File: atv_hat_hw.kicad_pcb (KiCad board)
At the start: 2 copper layers, 84.1 x 83.9 mm, 51 parts, among them J1 GPIO_CONNECTOR, J10 conn_01x02_labeled, J11 conn_01x02_labeled, J12 conn_01x02_labeled, J2 conn_01x02_labeled, J3 conn_01x02_labeled, J4 conn_01x02_labeled, J5 conn_01x02_labeled, J6 conn_01x02_labeled, J7 enc28j60_hanrun, J8 conn_01x02_labeled, J9 conn_01x02_labeled, Q1 Q_NMOS_GDS, Q2 Q_NMOS_GDS, Q3 Q_NMOS_GDS, Q4 Q_NMOS_GDS, Q5 Q_NMOS_GDS, Q6 Q_NMOS_GDS, Q7 Q_NMOS_GDS, Q8 Q_NMOS_GDS, Q9 Q_NMOS_GDS

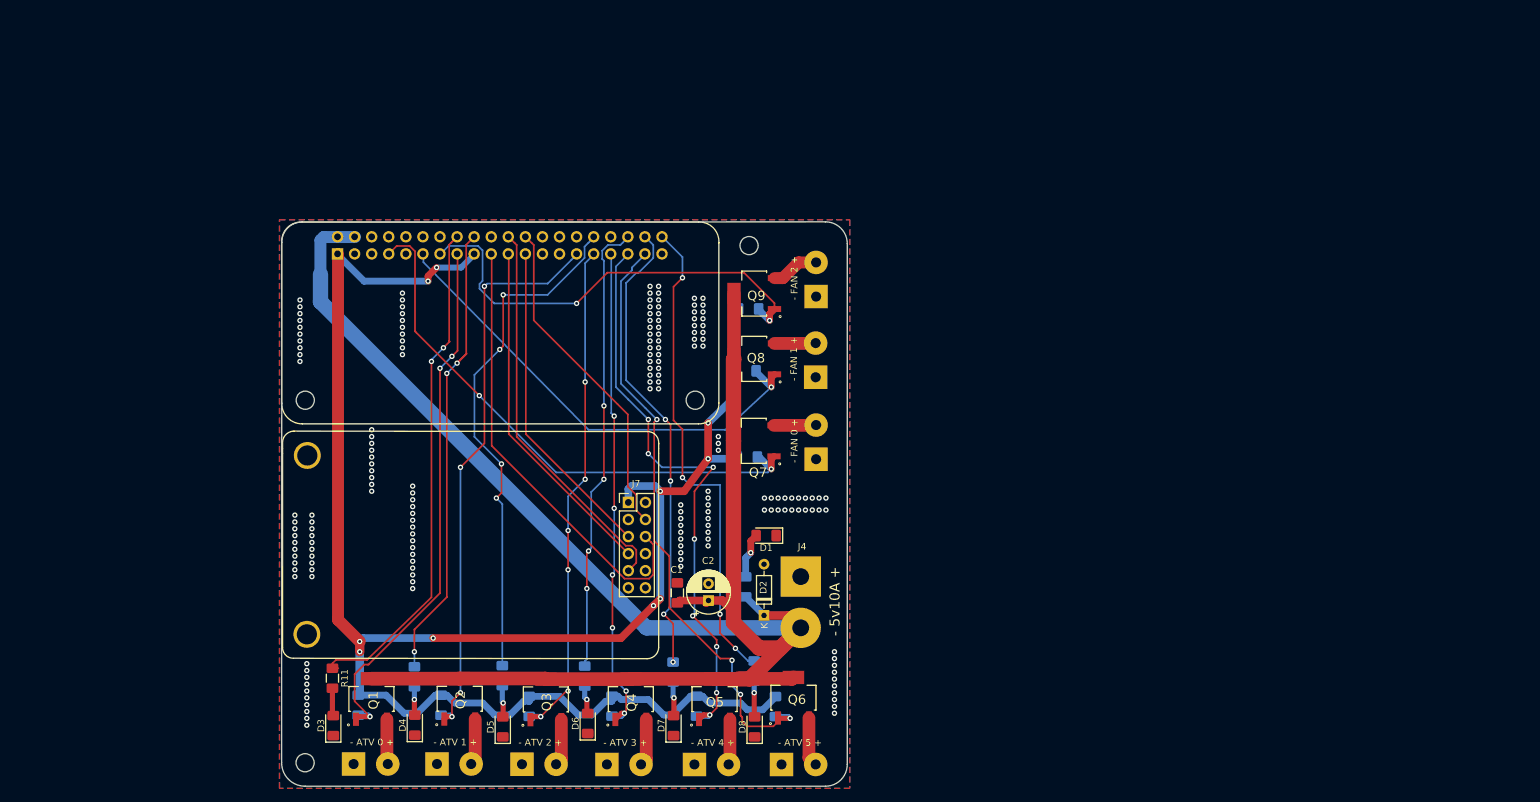
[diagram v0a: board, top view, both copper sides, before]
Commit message: plus board ready for routing
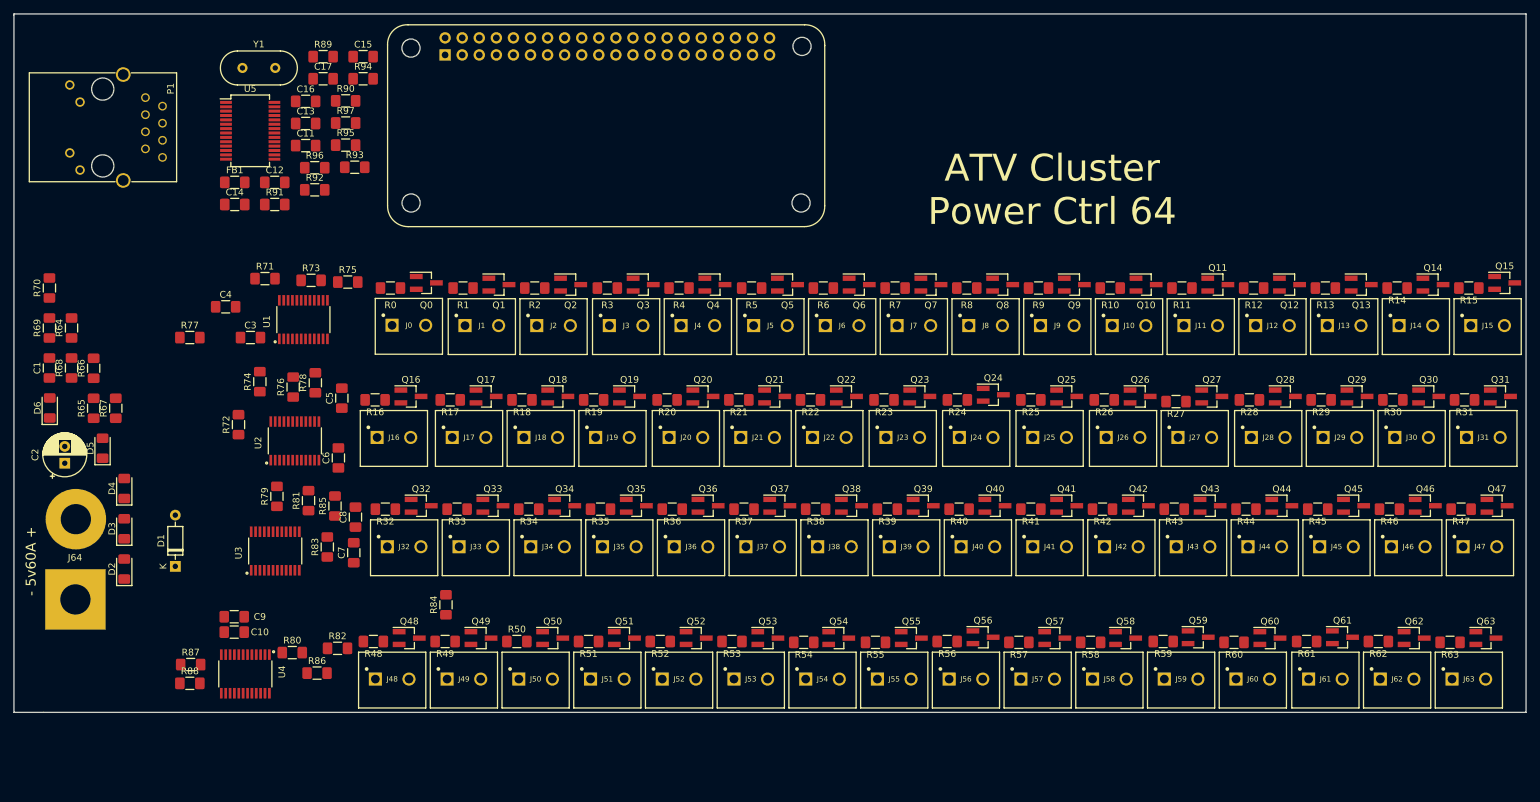
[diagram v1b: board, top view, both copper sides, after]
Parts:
- removed D7, D8: Green, LED_SMD:LED_1206_3216Metric_Pad1.42x1.75mm_HandSolder
- removed the H4 at (90.6, 129.6)
- added C10: 10u, Capacitor_SMD:C_1206_3216Metric_Pad1.42x1.75mm_HandSolder, F.Cu at (80.0, 107.9)
- added C11: 100n, Capacitor_SMD:C_1206_3216Metric_Pad1.42x1.75mm_HandSolder, F.Cu at (90.6, 37.8)
- added C12: 30p, Capacitor_SMD:C_1206_3216Metric_Pad1.42x1.75mm_HandSolder, F.Cu at (86.0, 43.3)
- added C13: 30p, Capacitor_SMD:C_1206_3216Metric_Pad1.42x1.75mm_HandSolder, F.Cu at (90.6, 34.5)
- added C14: 10u, Capacitor_SMD:C_1206_3216Metric_Pad1.42x1.75mm_HandSolder, F.Cu at (80.1, 46.6)
- added C15: 100n, Capacitor_SMD:C_1206_3216Metric_Pad1.42x1.75mm_HandSolder, F.Cu at (99.2, 24.6)
- added C16: 100n, Capacitor_SMD:C_1206_3216Metric_Pad1.42x1.75mm_HandSolder, F.Cu at (90.6, 31.2)
- added C17: 10u, Capacitor_SMD:C_1206_3216Metric_Pad1.42x1.75mm_HandSolder, F.Cu at (93.2, 27.9)
- added C3: 100n, Capacitor_SMD:C_1206_3216Metric_Pad1.42x1.75mm_HandSolder, F.Cu at (82.4, 66.4)
- added C4: 10u, Capacitor_SMD:C_1206_3216Metric_Pad1.42x1.75mm_HandSolder, F.Cu at (78.7, 61.8)
- added C5: 100n, Capacitor_SMD:C_1206_3216Metric_Pad1.42x1.75mm_HandSolder, F.Cu at (96.0, 75.4)
- added C6: 10u, Capacitor_SMD:C_1206_3216Metric_Pad1.42x1.75mm_HandSolder, F.Cu at (95.5, 84.3)
- added C7: 100n, Capacitor_SMD:C_1206_3216Metric_Pad1.42x1.75mm_HandSolder, F.Cu at (97.8, 98.4)
- added C8: 10u, Capacitor_SMD:C_1206_3216Metric_Pad1.42x1.75mm_HandSolder, F.Cu at (98.0, 93.1)
- added C9: 100n, Capacitor_SMD:C_1206_3216Metric_Pad1.42x1.75mm_HandSolder, F.Cu at (80.0, 110.2)
- added FB1: 80mA, Inductor_SMD:L_1206_3216Metric_Pad1.42x1.75mm_HandSolder, F.Cu at (80.1, 43.3)
- added H1: MountingHole, lib:MountingHole_2.7mm_M2.5_uHAT_RPi, F.Cu at (106.3, 23.3)
- added J0: phoenix_1935161, lib:PHOENIX_1935161, F.Cu at (106.0, 64.6)
- added J13: phoenix_1935161, lib:PHOENIX_1935161, F.Cu at (245.1, 64.6)
- added J14: phoenix_1935161, lib:PHOENIX_1935161, F.Cu at (255.8, 64.6)
- added J15: phoenix_1935161, lib:PHOENIX_1935161, F.Cu at (266.4, 64.6)
- added J16: phoenix_1935161, lib:PHOENIX_1935161, F.Cu at (103.8, 81.2)
- added J17: phoenix_1935161, lib:PHOENIX_1935161, F.Cu at (114.9, 81.2)
- added J18: phoenix_1935161, lib:PHOENIX_1935161, F.Cu at (125.6, 81.2)
- added J19: phoenix_1935161, lib:PHOENIX_1935161, F.Cu at (136.3, 81.2)
- added J20: phoenix_1935161, lib:PHOENIX_1935161, F.Cu at (147.2, 81.2)
- added J21: phoenix_1935161, lib:PHOENIX_1935161, F.Cu at (157.9, 81.2)
- added J22: phoenix_1935161, lib:PHOENIX_1935161, F.Cu at (168.5, 81.2)
- added J23: phoenix_1935161, lib:PHOENIX_1935161, F.Cu at (179.5, 81.2)
- added J24: phoenix_1935161, lib:PHOENIX_1935161, F.Cu at (190.4, 81.2)
- added J25: phoenix_1935161, lib:PHOENIX_1935161, F.Cu at (201.3, 81.2)
- added J26: phoenix_1935161, lib:PHOENIX_1935161, F.Cu at (212.2, 81.2)
- added J27: phoenix_1935161, lib:PHOENIX_1935161, F.Cu at (222.9, 81.2)
- added J28: phoenix_1935161, lib:PHOENIX_1935161, F.Cu at (233.8, 81.2)
- added J29: phoenix_1935161, lib:PHOENIX_1935161, F.Cu at (244.5, 81.2)
- added J30: phoenix_1935161, lib:PHOENIX_1935161, F.Cu at (255.1, 81.2)
- added J31: phoenix_1935161, lib:PHOENIX_1935161, F.Cu at (265.8, 81.2)
- added J32: phoenix_1935161, lib:PHOENIX_1935161, F.Cu at (105.3, 97.5)
- added J33: phoenix_1935161, lib:PHOENIX_1935161, F.Cu at (116.0, 97.5)
- added J34: phoenix_1935161, lib:PHOENIX_1935161, F.Cu at (126.6, 97.5)
- added J35: phoenix_1935161, lib:PHOENIX_1935161, F.Cu at (137.3, 97.5)
- added J36: phoenix_1935161, lib:PHOENIX_1935161, F.Cu at (148.0, 97.5)
- added J37: phoenix_1935161, lib:PHOENIX_1935161, F.Cu at (158.6, 97.5)
- added J38: phoenix_1935161, lib:PHOENIX_1935161, F.Cu at (169.3, 97.5)
- added J39: phoenix_1935161, lib:PHOENIX_1935161, F.Cu at (180.0, 97.5)
- added J40: phoenix_1935161, lib:PHOENIX_1935161, F.Cu at (190.6, 97.5)
- added J41: phoenix_1935161, lib:PHOENIX_1935161, F.Cu at (201.3, 97.5)
- added J42: phoenix_1935161, lib:PHOENIX_1935161, F.Cu at (212.0, 97.5)
- added J43: phoenix_1935161, lib:PHOENIX_1935161, F.Cu at (222.6, 97.5)
- added J44: phoenix_1935161, lib:PHOENIX_1935161, F.Cu at (233.3, 97.5)
- added J45: phoenix_1935161, lib:PHOENIX_1935161, F.Cu at (244.0, 97.5)
- added J46: phoenix_1935161, lib:PHOENIX_1935161, F.Cu at (254.6, 97.5)
- added J47: phoenix_1935161, lib:PHOENIX_1935161, F.Cu at (265.3, 97.5)
- added J48: phoenix_1935161, lib:PHOENIX_1935161, F.Cu at (103.5, 117.2)
- added J49: phoenix_1935161, lib:PHOENIX_1935161, F.Cu at (114.2, 117.2)
- added J50: phoenix_1935161, lib:PHOENIX_1935161, F.Cu at (124.8, 117.2)
- added J51: phoenix_1935161, lib:PHOENIX_1935161, F.Cu at (135.5, 117.2)
- added J52: phoenix_1935161, lib:PHOENIX_1935161, F.Cu at (146.2, 117.2)
- added J53: phoenix_1935161, lib:PHOENIX_1935161, F.Cu at (156.8, 117.2)
- added J54: phoenix_1935161, lib:PHOENIX_1935161, F.Cu at (167.5, 117.2)
- added J55: phoenix_1935161, lib:PHOENIX_1935161, F.Cu at (178.2, 117.2)
- added J56: phoenix_1935161, lib:PHOENIX_1935161, F.Cu at (188.8, 117.2)
- added J57: phoenix_1935161, lib:PHOENIX_1935161, F.Cu at (199.5, 117.2)
- added J58: phoenix_1935161, lib:PHOENIX_1935161, F.Cu at (210.2, 117.2)
- added J59: phoenix_1935161, lib:PHOENIX_1935161, F.Cu at (220.9, 117.2)
- added J60: phoenix_1935161, lib:PHOENIX_1935161, F.Cu at (231.5, 117.2)
- added J61: phoenix_1935161, lib:PHOENIX_1935161, F.Cu at (242.3, 117.2)
- added J62: phoenix_1935161, lib:PHOENIX_1935161, F.Cu at (253.0, 117.2)
- added J63: phoenix_1935161, lib:PHOENIX_1935161, F.Cu at (263.7, 117.2)
- added J64: phoenix_1935161, lib:SolderWirePad_1x02_P9.0mm_Drill4.5mm, F.Cu at (56.5, 105.3)
- added J65: GPIO_CONNECTOR, lib:PinSocket_2x20_P2.54mm_Vertical_Centered_Anchor, B.Cu at (135.5, 23.1)
- added P1: RB1-125BAG1A, WIZNET_RB1-125BAG1A, F.Cu at (60.5, 35.1)
- added Q0: Q_NMOS_GSD, Package_TO_SOT_SMD:SOT-23_Handsoldering, F.Cu at (108.6, 58.2)
- added Q10: Q_NMOS_GSD, Package_TO_SOT_SMD:SOT-23_Handsoldering, F.Cu at (215.6, 58.5)
- added Q11: Q_NMOS_GSD, Package_TO_SOT_SMD:SOT-23_Handsoldering, F.Cu at (226.3, 58.5)
- added Q12: Q_NMOS_GSD, Package_TO_SOT_SMD:SOT-23_Handsoldering, F.Cu at (237.0, 58.5)
- added Q13: Q_NMOS_GSD, Package_TO_SOT_SMD:SOT-23_Handsoldering, F.Cu at (247.7, 58.5)
- added Q14: Q_NMOS_GSD, Package_TO_SOT_SMD:SOT-23_Handsoldering, F.Cu at (258.3, 58.5)
- added Q15: Q_NMOS_GSD, Package_TO_SOT_SMD:SOT-23_Handsoldering, F.Cu at (269.0, 58.2)
- added Q16: Q_NMOS_GSD, Package_TO_SOT_SMD:SOT-23_Handsoldering, F.Cu at (106.3, 75.1)
- added Q17: Q_NMOS_GSD, Package_TO_SOT_SMD:SOT-23_Handsoldering, F.Cu at (117.5, 75.1)
- added Q18: Q_NMOS_GSD, Package_TO_SOT_SMD:SOT-23_Handsoldering, F.Cu at (128.1, 75.1)
- added Q19: Q_NMOS_GSD, Package_TO_SOT_SMD:SOT-23_Handsoldering, F.Cu at (138.8, 75.1)
- added Q20: Q_NMOS_GSD, Package_TO_SOT_SMD:SOT-23_Handsoldering, F.Cu at (149.7, 75.1)
- added Q21: Q_NMOS_GSD, Package_TO_SOT_SMD:SOT-23_Handsoldering, F.Cu at (160.4, 75.1)
- added Q22: Q_NMOS_GSD, Package_TO_SOT_SMD:SOT-23_Handsoldering, F.Cu at (171.1, 75.1)
- added Q23: Q_NMOS_GSD, Package_TO_SOT_SMD:SOT-23_Handsoldering, F.Cu at (182.0, 75.1)
- added Q24: Q_NMOS_GSD, Package_TO_SOT_SMD:SOT-23_Handsoldering, F.Cu at (192.9, 74.9)
- added Q25: Q_NMOS_GSD, Package_TO_SOT_SMD:SOT-23_Handsoldering, F.Cu at (203.8, 75.1)
- added Q26: Q_NMOS_GSD, Package_TO_SOT_SMD:SOT-23_Handsoldering, F.Cu at (214.8, 75.1)
- added Q27: Q_NMOS_GSD, Package_TO_SOT_SMD:SOT-23_Handsoldering, F.Cu at (225.4, 75.1)
- added Q28: Q_NMOS_GSD, Package_TO_SOT_SMD:SOT-23_Handsoldering, F.Cu at (236.3, 75.1)
- added Q29: Q_NMOS_GSD, Package_TO_SOT_SMD:SOT-23_Handsoldering, F.Cu at (247.0, 75.1)
- added Q30: Q_NMOS_GSD, Package_TO_SOT_SMD:SOT-23_Handsoldering, F.Cu at (257.7, 75.1)
- added Q31: Q_NMOS_GSD, Package_TO_SOT_SMD:SOT-23_Handsoldering, F.Cu at (268.4, 75.1)
- added Q32: Q_NMOS_GSD, Package_TO_SOT_SMD:SOT-23_Handsoldering, F.Cu at (107.8, 91.4)
- added Q33: Q_NMOS_GSD, Package_TO_SOT_SMD:SOT-23_Handsoldering, F.Cu at (118.5, 91.4)
- added Q34: Q_NMOS_GSD, Package_TO_SOT_SMD:SOT-23_Handsoldering, F.Cu at (129.2, 91.4)
- added Q35: Q_NMOS_GSD, Package_TO_SOT_SMD:SOT-23_Handsoldering, F.Cu at (139.8, 91.4)
- added Q36: Q_NMOS_GSD, Package_TO_SOT_SMD:SOT-23_Handsoldering, F.Cu at (150.5, 91.4)
- added Q37: Q_NMOS_GSD, Package_TO_SOT_SMD:SOT-23_Handsoldering, F.Cu at (161.2, 91.4)
- added Q38: Q_NMOS_GSD, Package_TO_SOT_SMD:SOT-23_Handsoldering, F.Cu at (171.8, 91.4)
- added Q39: Q_NMOS_GSD, Package_TO_SOT_SMD:SOT-23_Handsoldering, F.Cu at (182.5, 91.4)
- added Q40: Q_NMOS_GSD, Package_TO_SOT_SMD:SOT-23_Handsoldering, F.Cu at (193.2, 91.4)
- added Q41: Q_NMOS_GSD, Package_TO_SOT_SMD:SOT-23_Handsoldering, F.Cu at (203.8, 91.4)
- added Q42: Q_NMOS_GSD, Package_TO_SOT_SMD:SOT-23_Handsoldering, F.Cu at (214.5, 91.4)
- added Q43: Q_NMOS_GSD, Package_TO_SOT_SMD:SOT-23_Handsoldering, F.Cu at (225.2, 91.4)
- added Q44: Q_NMOS_GSD, Package_TO_SOT_SMD:SOT-23_Handsoldering, F.Cu at (235.8, 91.4)
- added Q45: Q_NMOS_GSD, Package_TO_SOT_SMD:SOT-23_Handsoldering, F.Cu at (246.5, 91.4)
- added Q46: Q_NMOS_GSD, Package_TO_SOT_SMD:SOT-23_Handsoldering, F.Cu at (257.2, 91.4)
- added Q47: Q_NMOS_GSD, Package_TO_SOT_SMD:SOT-23_Handsoldering, F.Cu at (267.8, 91.4)
- added Q48: Q_NMOS_GSD, Package_TO_SOT_SMD:SOT-23_Handsoldering, F.Cu at (106.0, 111.1)
- added Q49: Q_NMOS_GSD, Package_TO_SOT_SMD:SOT-23_Handsoldering, F.Cu at (116.7, 111.1)
- added Q50: Q_NMOS_GSD, Package_TO_SOT_SMD:SOT-23_Handsoldering, F.Cu at (127.4, 111.1)
- added Q51: Q_NMOS_GSD, Package_TO_SOT_SMD:SOT-23_Handsoldering, F.Cu at (138.1, 111.1)
- added Q52: Q_NMOS_GSD, Package_TO_SOT_SMD:SOT-23_Handsoldering, F.Cu at (148.7, 111.1)
- added Q53: Q_NMOS_GSD, Package_TO_SOT_SMD:SOT-23_Handsoldering, F.Cu at (159.4, 111.1)
- added Q54: Q_NMOS_GSD, Package_TO_SOT_SMD:SOT-23_Handsoldering, F.Cu at (169.9, 111.1)
- added Q55: Q_NMOS_GSD, Package_TO_SOT_SMD:SOT-23_Handsoldering, F.Cu at (180.7, 111.1)
- added Q56: Q_NMOS_GSD, Package_TO_SOT_SMD:SOT-23_Handsoldering, F.Cu at (191.4, 111.0)
- added Q57: Q_NMOS_GSD, Package_TO_SOT_SMD:SOT-23_Handsoldering, F.Cu at (202.1, 111.1)
- added Q58: Q_NMOS_GSD, Package_TO_SOT_SMD:SOT-23_Handsoldering, F.Cu at (212.6, 111.1)
- added Q59: Q_NMOS_GSD, Package_TO_SOT_SMD:SOT-23_Handsoldering, F.Cu at (223.4, 111.0)
- added Q60: Q_NMOS_GSD, Package_TO_SOT_SMD:SOT-23_Handsoldering, F.Cu at (234.1, 111.1)
- added Q61: Q_NMOS_GSD, Package_TO_SOT_SMD:SOT-23_Handsoldering, F.Cu at (244.9, 111.0)
- added Q62: Q_NMOS_GSD, Package_TO_SOT_SMD:SOT-23_Handsoldering, F.Cu at (255.5, 111.1)
- added Q63: Q_NMOS_GSD, Package_TO_SOT_SMD:SOT-23_Handsoldering, F.Cu at (266.2, 111.1)
- added R0: 10k, Resistor_SMD:R_1206_3216Metric_Pad1.42x1.75mm_HandSolder, F.Cu at (103.3, 59.0)
- added R17: 10k, Resistor_SMD:R_1206_3216Metric_Pad1.42x1.75mm_HandSolder, F.Cu at (112.1, 75.6)
- added R18: 10k, Resistor_SMD:R_1206_3216Metric_Pad1.42x1.75mm_HandSolder, F.Cu at (122.8, 75.6)
- added R19: 10k, Resistor_SMD:R_1206_3216Metric_Pad1.42x1.75mm_HandSolder, F.Cu at (133.5, 75.6)
- added R20: 10k, Resistor_SMD:R_1206_3216Metric_Pad1.42x1.75mm_HandSolder, F.Cu at (144.4, 75.6)
- added R21: 10k, Resistor_SMD:R_1206_3216Metric_Pad1.42x1.75mm_HandSolder, F.Cu at (155.1, 75.6)
- added R22: 10k, Resistor_SMD:R_1206_3216Metric_Pad1.42x1.75mm_HandSolder, F.Cu at (165.7, 75.6)
- added R23: 10k, Resistor_SMD:R_1206_3216Metric_Pad1.42x1.75mm_HandSolder, F.Cu at (176.7, 75.6)
- added R24: 10k, Resistor_SMD:R_1206_3216Metric_Pad1.42x1.75mm_HandSolder, F.Cu at (187.6, 75.6)
- added R25: 10k, Resistor_SMD:R_1206_3216Metric_Pad1.42x1.75mm_HandSolder, F.Cu at (198.5, 75.6)
- added R26: 10k, Resistor_SMD:R_1206_3216Metric_Pad1.42x1.75mm_HandSolder, F.Cu at (209.4, 75.6)
- added R27: 10k, Resistor_SMD:R_1206_3216Metric_Pad1.42x1.75mm_HandSolder, F.Cu at (220.1, 75.9)
- added R28: 10k, Resistor_SMD:R_1206_3216Metric_Pad1.42x1.75mm_HandSolder, F.Cu at (231.0, 75.6)
- added R29: 10k, Resistor_SMD:R_1206_3216Metric_Pad1.42x1.75mm_HandSolder, F.Cu at (241.7, 75.6)
- added R30: 10k, Resistor_SMD:R_1206_3216Metric_Pad1.42x1.75mm_HandSolder, F.Cu at (252.3, 75.6)
- added R31: 10k, Resistor_SMD:R_1206_3216Metric_Pad1.42x1.75mm_HandSolder, F.Cu at (263.0, 75.6)
- added R32: 10k, Resistor_SMD:R_1206_3216Metric_Pad1.42x1.75mm_HandSolder, F.Cu at (102.5, 91.9)
- added R33: 10k, Resistor_SMD:R_1206_3216Metric_Pad1.42x1.75mm_HandSolder, F.Cu at (113.2, 91.9)
- added R34: 10k, Resistor_SMD:R_1206_3216Metric_Pad1.42x1.75mm_HandSolder, F.Cu at (123.8, 91.9)
- added R35: 10k, Resistor_SMD:R_1206_3216Metric_Pad1.42x1.75mm_HandSolder, F.Cu at (134.5, 91.9)
- added R36: 10k, Resistor_SMD:R_1206_3216Metric_Pad1.42x1.75mm_HandSolder, F.Cu at (145.2, 91.9)
- added R37: 10k, Resistor_SMD:R_1206_3216Metric_Pad1.42x1.75mm_HandSolder, F.Cu at (155.8, 91.9)
- added R38: 10k, Resistor_SMD:R_1206_3216Metric_Pad1.42x1.75mm_HandSolder, F.Cu at (166.5, 91.9)
- added R39: 10k, Resistor_SMD:R_1206_3216Metric_Pad1.42x1.75mm_HandSolder, F.Cu at (177.2, 91.9)
- added R40: 10k, Resistor_SMD:R_1206_3216Metric_Pad1.42x1.75mm_HandSolder, F.Cu at (187.8, 91.9)
- added R41: 10k, Resistor_SMD:R_1206_3216Metric_Pad1.42x1.75mm_HandSolder, F.Cu at (198.5, 91.9)
- added R42: 10k, Resistor_SMD:R_1206_3216Metric_Pad1.42x1.75mm_HandSolder, F.Cu at (209.2, 91.9)
- added R43: 10k, Resistor_SMD:R_1206_3216Metric_Pad1.42x1.75mm_HandSolder, F.Cu at (219.8, 91.9)
- added R44: 10k, Resistor_SMD:R_1206_3216Metric_Pad1.42x1.75mm_HandSolder, F.Cu at (230.5, 91.9)
- added R45: 10k, Resistor_SMD:R_1206_3216Metric_Pad1.42x1.75mm_HandSolder, F.Cu at (241.2, 91.9)
- added R46: 10k, Resistor_SMD:R_1206_3216Metric_Pad1.42x1.75mm_HandSolder, F.Cu at (251.8, 91.9)
- added R47: 10k, Resistor_SMD:R_1206_3216Metric_Pad1.42x1.75mm_HandSolder, F.Cu at (262.5, 91.9)
- added R48: 10k, Resistor_SMD:R_1206_3216Metric_Pad1.42x1.75mm_HandSolder, F.Cu at (100.7, 111.6)
- added R49: 10k, Resistor_SMD:R_1206_3216Metric_Pad1.42x1.75mm_HandSolder, F.Cu at (111.4, 111.6)
- added R50: 10k, Resistor_SMD:R_1206_3216Metric_Pad1.42x1.75mm_HandSolder, F.Cu at (122.0, 111.6)
- added R51: 10k, Resistor_SMD:R_1206_3216Metric_Pad1.42x1.75mm_HandSolder, F.Cu at (132.7, 111.6)
- added R52: 10k, Resistor_SMD:R_1206_3216Metric_Pad1.42x1.75mm_HandSolder, F.Cu at (143.4, 111.6)
- added R53: 10k, Resistor_SMD:R_1206_3216Metric_Pad1.42x1.75mm_HandSolder, F.Cu at (154.1, 111.6)
- added R54: 10k, Resistor_SMD:R_1206_3216Metric_Pad1.42x1.75mm_HandSolder, F.Cu at (164.7, 111.7)
- added R55: 10k, Resistor_SMD:R_1206_3216Metric_Pad1.42x1.75mm_HandSolder, F.Cu at (175.4, 111.7)
- added R56: 10k, Resistor_SMD:R_1206_3216Metric_Pad1.42x1.75mm_HandSolder, F.Cu at (186.1, 111.6)
- added R57: 10k, Resistor_SMD:R_1206_3216Metric_Pad1.42x1.75mm_HandSolder, F.Cu at (196.7, 111.7)
- added R58: 10k, Resistor_SMD:R_1206_3216Metric_Pad1.42x1.75mm_HandSolder, F.Cu at (207.4, 111.7)
- added R59: 10k, Resistor_SMD:R_1206_3216Metric_Pad1.42x1.75mm_HandSolder, F.Cu at (218.2, 111.6)
- added R60: 10k, Resistor_SMD:R_1206_3216Metric_Pad1.42x1.75mm_HandSolder, F.Cu at (228.7, 111.7)
- added R61: 10k, Resistor_SMD:R_1206_3216Metric_Pad1.42x1.75mm_HandSolder, F.Cu at (239.5, 111.6)
- added R62: 10k, Resistor_SMD:R_1206_3216Metric_Pad1.42x1.75mm_HandSolder, F.Cu at (250.2, 111.6)
- added R63: 10k, Resistor_SMD:R_1206_3216Metric_Pad1.42x1.75mm_HandSolder, F.Cu at (260.9, 111.7)
- added R64: 220, Resistor_SMD:R_1206_3216Metric_Pad1.42x1.75mm_HandSolder, F.Cu at (55.8, 65.0)
- added R65: 10k, Resistor_SMD:R_1206_3216Metric_Pad1.42x1.75mm_HandSolder, F.Cu at (59.1, 76.9)
- added R66: 10k, Resistor_SMD:R_1206_3216Metric_Pad1.42x1.75mm_HandSolder, F.Cu at (59.1, 70.9)
- added R67: 220, Resistor_SMD:R_1206_3216Metric_Pad1.42x1.75mm_HandSolder, F.Cu at (62.4, 76.9)
- added R68: 220, Resistor_SMD:R_1206_3216Metric_Pad1.42x1.75mm_HandSolder, F.Cu at (55.8, 70.9)
- added R69: 220, Resistor_SMD:R_1206_3216Metric_Pad1.42x1.75mm_HandSolder, F.Cu at (52.5, 65.0)
- added R70: 220, Resistor_SMD:R_1206_3216Metric_Pad1.42x1.75mm_HandSolder, F.Cu at (52.5, 59.0)
- added R71: 10k, Resistor_SMD:R_1206_3216Metric_Pad1.42x1.75mm_HandSolder, F.Cu at (84.6, 57.6)
- added R72: 10k, Resistor_SMD:R_1206_3216Metric_Pad1.42x1.75mm_HandSolder, F.Cu at (80.6, 79.3)
- added R73: 10k, Resistor_SMD:R_1206_3216Metric_Pad1.42x1.75mm_HandSolder, F.Cu at (91.4, 57.9)
- added R74: 10k, Resistor_SMD:R_1206_3216Metric_Pad1.42x1.75mm_HandSolder, F.Cu at (83.8, 72.9)
- added R75: 10k, Resistor_SMD:R_1206_3216Metric_Pad1.42x1.75mm_HandSolder, F.Cu at (96.9, 58.1)
- added R76: 10k, Resistor_SMD:R_1206_3216Metric_Pad1.42x1.75mm_HandSolder, F.Cu at (88.8, 73.7)
- added R77: 10k, Resistor_SMD:R_1206_3216Metric_Pad1.42x1.75mm_HandSolder, F.Cu at (73.4, 66.4)
- added R78: 10k, Resistor_SMD:R_1206_3216Metric_Pad1.42x1.75mm_HandSolder, F.Cu at (92.1, 73.1)
- added R79: 10k, Resistor_SMD:R_1206_3216Metric_Pad1.42x1.75mm_HandSolder, F.Cu at (86.4, 90.0)
- added R80: 10k, Resistor_SMD:R_1206_3216Metric_Pad1.42x1.75mm_HandSolder, F.Cu at (88.6, 113.2)
- added R81: 10k, Resistor_SMD:R_1206_3216Metric_Pad1.42x1.75mm_HandSolder, F.Cu at (91.1, 90.6)
- added R82: 10k, Resistor_SMD:R_1206_3216Metric_Pad1.42x1.75mm_HandSolder, F.Cu at (95.4, 112.6)
- added R83: 10k, Resistor_SMD:R_1206_3216Metric_Pad1.42x1.75mm_HandSolder, F.Cu at (93.9, 97.5)
- added R84: 10k, Resistor_SMD:R_1206_3216Metric_Pad1.42x1.75mm_HandSolder, F.Cu at (111.5, 106.1)
- added R85: 10k, Resistor_SMD:R_1206_3216Metric_Pad1.42x1.75mm_HandSolder, F.Cu at (95.0, 91.4)
- added R86: 10k, Resistor_SMD:R_1206_3216Metric_Pad1.42x1.75mm_HandSolder, F.Cu at (92.3, 116.3)
- added R87: 10k, Resistor_SMD:R_1206_3216Metric_Pad1.42x1.75mm_HandSolder, F.Cu at (73.5, 115.0)
- added R88: 10k, Resistor_SMD:R_1206_3216Metric_Pad1.42x1.75mm_HandSolder, F.Cu at (73.4, 117.8)
- added R89: 10k, Resistor_SMD:R_1206_3216Metric_Pad1.42x1.75mm_HandSolder, F.Cu at (93.2, 24.6)
- added R90: 10k, Resistor_SMD:R_1206_3216Metric_Pad1.42x1.75mm_HandSolder, F.Cu at (96.6, 31.2)
- added R91: 10k, Resistor_SMD:R_1206_3216Metric_Pad1.42x1.75mm_HandSolder, F.Cu at (86.0, 46.6)
- added R92: 10k, Resistor_SMD:R_1206_3216Metric_Pad1.42x1.75mm_HandSolder, F.Cu at (92.0, 44.4)
- added R93: 49.9, Resistor_SMD:R_1206_3216Metric_Pad1.42x1.75mm_HandSolder, F.Cu at (97.9, 41.0)
- added R94: 49.9, Resistor_SMD:R_1206_3216Metric_Pad1.42x1.75mm_HandSolder, F.Cu at (99.2, 27.9)
- added R95: 49.9, Resistor_SMD:R_1206_3216Metric_Pad1.42x1.75mm_HandSolder, F.Cu at (96.6, 37.8)
- added R96: 2.32k, Resistor_SMD:R_1206_3216Metric_Pad1.42x1.75mm_HandSolder, F.Cu at (92.0, 41.1)
- added R97: 49.9, Resistor_SMD:R_1206_3216Metric_Pad1.42x1.75mm_HandSolder, F.Cu at (96.6, 34.5)
- added U1: PCA9552PW,118, lib:SOP65P640X110-24N, F.Cu at (90.3, 63.7)
- added U2: PCA9552PW,118, lib:SOP65P640X110-24N, F.Cu at (89.0, 81.7)
- added U3: PCA9552PW,118, lib:SOP65P640X110-24N, F.Cu at (86.1, 98.1)
- added U4: PCA9552PW,118, lib:SOP65P640X110-24N, F.Cu at (81.7, 116.4)
- added U5: ENC28J60x-SS, Package_SO:SSOP-28_5.3x10.2mm_P0.65mm, F.Cu at (82.4, 35.6)
- added Y1: Crystal, Crystal:Crystal_HC49-4H_Vertical, F.Cu at (81.2, 26.3)
- D1: value Blue -> 5.6v; footprint LED_SMD:LED_1206_3216Metric_Pad1.42x1.75mm_HandSolder -> Diode_THT:D_DO-35_SOD27_P7.62mm_Horizontal
- D2: value 5.6v -> Blue; footprint Diode_THT:D_DO-35_SOD27_P7.62mm_Horizontal -> LED_SMD:LED_1206_3216Metric_Pad1.42x1.75mm_HandSolder
- J1: value GPIO_CONNECTOR -> phoenix_1935161; footprint lib:PinSocket_2x20_P2.54mm_Vertical_Centered_Anchor -> lib:PHOENIX_1935161; moved to F.Cu
- J10, J11, J12, J2, J3, J5, J6, J8, J9: value conn_01x02_labeled -> phoenix_1935161; footprint lib:SolderWirePad_1x02_P5.08mm_Drill1.5mm_labeled -> lib:PHOENIX_1935161
- J4: value conn_01x02_labeled -> phoenix_1935161; footprint Connector_Wire:SolderWirePad_1x02_P7.62mm_Drill2.5mm -> lib:PHOENIX_1935161
- J7: value enc28j60_hanrun -> phoenix_1935161; footprint lib:enc28j60_hanrun -> lib:PHOENIX_1935161
- Q1, Q2, Q3, Q4, Q5, Q6, Q7, Q8, Q9: value Q_NMOS_GDS -> Q_NMOS_GSD; footprint lib:SOT230P700X180-3N -> Package_TO_SOT_SMD:SOT-23_Handsoldering
- R1, R10, R2, R4, R5, R6, R7, R8, R9: moved to F.Cu
- R11: value 220 -> 10k
- R12, R13, R14, R15, R16, R3: value 220 -> 10k; moved to F.Cu
- moved R11 139.1 mm to (221.0, 59.0), turned to 180 degrees
- moved R12 137.6 mm to (231.6, 59.0), turned to 180 degrees
- moved R13 135.3 mm to (242.3, 59.0), turned to 180 degrees
- moved R14 133.9 mm to (253.0, 59.0), turned to 180 degrees
- moved R15 131.4 mm to (263.7, 59.0), turned to 180 degrees
- moved C1 99.2 mm to (52.5, 70.9), turned to 90 degrees
- moved C2 97.9 mm to (54.8, 85.1)
- moved D2 95.4 mm to (63.7, 100.8)
- moved D6 92.8 mm to (52.6, 76.8)
- moved D1 88.0 mm to (71.2, 100.4), turned to 90 degrees
- moved J8 78.3 mm to (191.8, 64.6)
- moved J9 77.1 mm to (202.4, 64.6)
- moved J5 75.0 mm to (159.8, 64.6)
- moved J6 74.1 mm to (170.4, 64.6)
- moved D5 72.5 mm to (60.4, 82.8)
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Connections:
- D1 pad 1: GND -> +5V
- D1 pad 2: Net-(D1-Pad2) -> GND
- D2 pad 1: +5V -> GND
- D2 pad 2: GND -> Net-(D2-Pad2)
- J1 pad 1: +3V3 -> GND
- J1 pad 2: +5V -> Net-(J1-Pad2)
- J4 pad 2: +5V -> Net-(J4-Pad2)
- J7 pad 1: +3V3 -> GND
- J7 pad 2: GND -> Net-(J7-Pad2)
- Q1 pad 1: /ATV0_CTRL -> pwr_toggle_01
- Q1 pad 2: +5V -> Net-(J1-Pad2)
- Q1 pad 3: Net-(J2-Pad2) -> +5V
- Q2 pad 1: /ATV1_CTRL -> pwr_toggle_02
- Q2 pad 2: +5V -> Net-(J2-Pad2)
- Q2 pad 3: Net-(J3-Pad2) -> +5V
- Q3 pad 1: /ATV2_CTRL -> pwr_toggle_03
- Q3 pad 2: +5V -> Net-(J3-Pad2)
- Q3 pad 3: Net-(J5-Pad2) -> +5V
- Q4 pad 1: /ATV3_CTRL -> pwr_toggle_04
- Q4 pad 2: +5V -> Net-(J4-Pad2)
- Q4 pad 3: Net-(J6-Pad2) -> +5V
- Q5 pad 1: /ATV4_CTRL -> pwr_toggle_05
- Q5 pad 2: +5V -> Net-(J5-Pad2)
- Q5 pad 3: Net-(J8-Pad2) -> +5V
- Q6 pad 1: /ATV5_CTRL -> pwr_toggle_06
- Q6 pad 2: +5V -> Net-(J6-Pad2)
- Q6 pad 3: Net-(J9-Pad2) -> +5V
- Q7 pad 1: /FAN0_PWM -> pwr_toggle_07
- Q7 pad 2: +5V -> Net-(J7-Pad2)
- Q7 pad 3: Net-(J10-Pad2) -> +5V
- Q8 pad 1: /FAN1_PWM -> pwr_toggle_08
- Q8 pad 2: +5V -> Net-(J8-Pad2)
- Q8 pad 3: Net-(J11-Pad2) -> +5V
- Q9 pad 1: /FAN2_PWM -> pwr_toggle_09
- Q9 pad 2: +5V -> Net-(J9-Pad2)
- Q9 pad 3: Net-(J12-Pad2) -> +5V
- R1 pad 1: +3V3 -> pwr_toggle_01
- R1 pad 2: /ATV0_CTRL -> +3V3
- R10 pad 1: +3V3 -> pwr_toggle_10
- R10 pad 2: /FAN2_PWM -> +3V3
- R11 pad 1: /GPIO23_GEN4 -> pwr_toggle_11
- R11 pad 2: Net-(D3-Pad2) -> +3V3
- R12 pad 1: /GPIO24_GEN5 -> pwr_toggle_12
- R12 pad 2: Net-(D4-Pad2) -> +3V3
- R13 pad 1: /GPIO12 -> pwr_toggle_13
- R13 pad 2: Net-(D5-Pad2) -> +3V3
- R14 pad 1: /GPIO16 -> pwr_toggle_14
- R14 pad 2: Net-(D6-Pad2) -> +3V3
- R15 pad 1: /GPIO20 -> pwr_toggle_15
- R15 pad 2: Net-(D7-Pad2) -> +3V3
- R16 pad 1: /GPIO21 -> pwr_toggle_16
- R16 pad 2: Net-(D8-Pad2) -> +3V3
- R2 pad 1: +3V3 -> pwr_toggle_02
- R2 pad 2: /ATV1_CTRL -> +3V3
- R3 pad 1: +5V -> pwr_toggle_03
- R3 pad 2: Net-(D1-Pad2) -> +3V3
- R4 pad 1: +3V3 -> pwr_toggle_04
- R4 pad 2: /ATV2_CTRL -> +3V3
- R5 pad 1: +3V3 -> pwr_toggle_05
- R5 pad 2: /ATV3_CTRL -> +3V3
- R6 pad 1: +3V3 -> pwr_toggle_06
- R6 pad 2: /ATV4_CTRL -> +3V3
- R7 pad 1: +3V3 -> pwr_toggle_07
- R7 pad 2: /ATV5_CTRL -> +3V3
- R8 pad 1: +3V3 -> pwr_toggle_08
- R8 pad 2: /FAN0_PWM -> +3V3
- R9 pad 1: +3V3 -> pwr_toggle_09
- R9 pad 2: /FAN1_PWM -> +3V3
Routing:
- net +3V3: track 273.9 -> 0.00 mm, vias 10 -> 0
- net +5V: track 268.1 -> 0.00 mm
- net /ATV5_CTRL: track 90.4 -> 0.00 mm, vias 4 -> 0
- net /ATV4_CTRL: track 86.7 -> 0.00 mm, vias 8 -> 0
- net /ATV1_CTRL: track 84.8 -> 0.00 mm, vias 4 -> 0
- net /FAN0_PWM: track 83.4 -> 0.00 mm, vias 2 -> 0
- net /ATV0_CTRL: track 80.5 -> 0.00 mm, vias 3 -> 0
- net /GPIO12: track 77.4 -> 0.00 mm, vias 4 -> 0
- net /ATV2_CTRL: track 75.7 -> 0.00 mm, vias 6 -> 0
- net /GPIO23_GEN4: track 75.6 -> 0.00 mm, vias 2 -> 0
- net /ATV3_CTRL: track 73.3 -> 0.00 mm, vias 6 -> 0
- net /GPIO21: track 73.0 -> 0.00 mm, vias 4 -> 0
- net /FAN1_PWM: track 71.3 -> 0.00 mm, vias 1 -> 0
- net /GPIO24_GEN5: track 69.7 -> 0.00 mm, vias 3 -> 0
- net /GPIO20: track 69.3 -> 0.00 mm, vias 4 -> 0
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- removed copper zone on B.Cu, net GND
- removed copper zone on F.Cu, net GND
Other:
- board size 84.1 x 83.9 mm -> 224.9 x 103.9 mm
- board text added: "- 5v60A +"
- board text added: "ATV Cluster Power Ctrl 64"
- board text removed: "- 5v10A +"
- board text removed: "ATV Cluster Power Ctrl"
